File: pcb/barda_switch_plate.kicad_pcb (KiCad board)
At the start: 2 copper layers, 228.6 x 76.2 mm, 4 parts

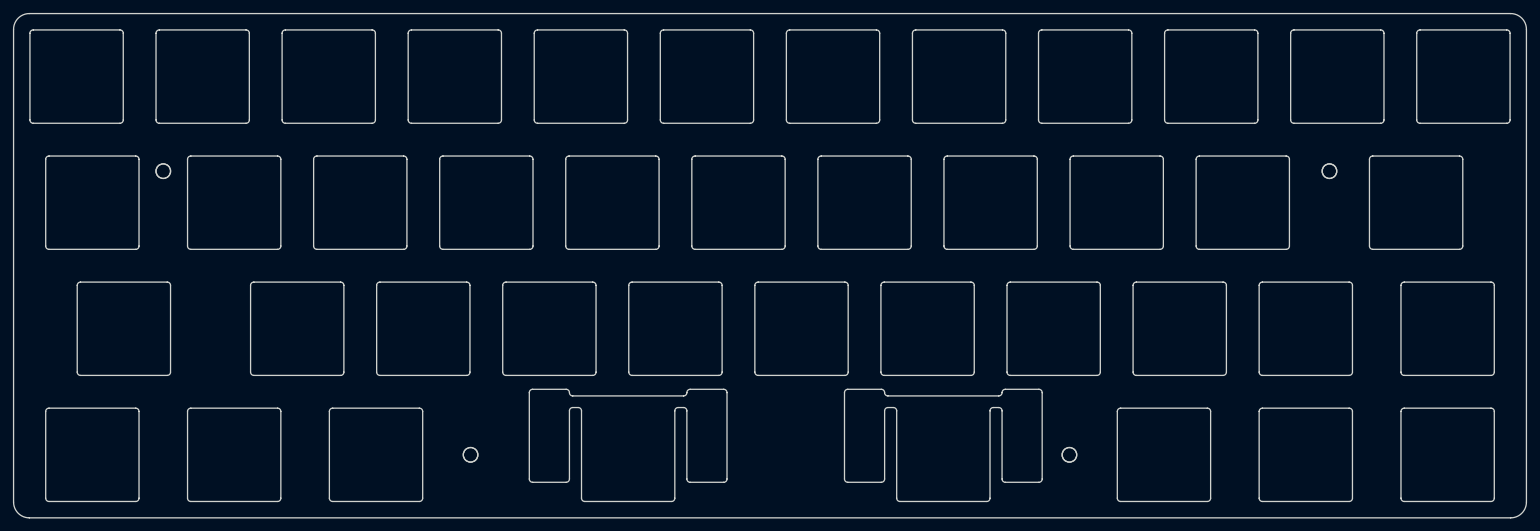
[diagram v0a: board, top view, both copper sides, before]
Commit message: Update Barda case and PCB designs
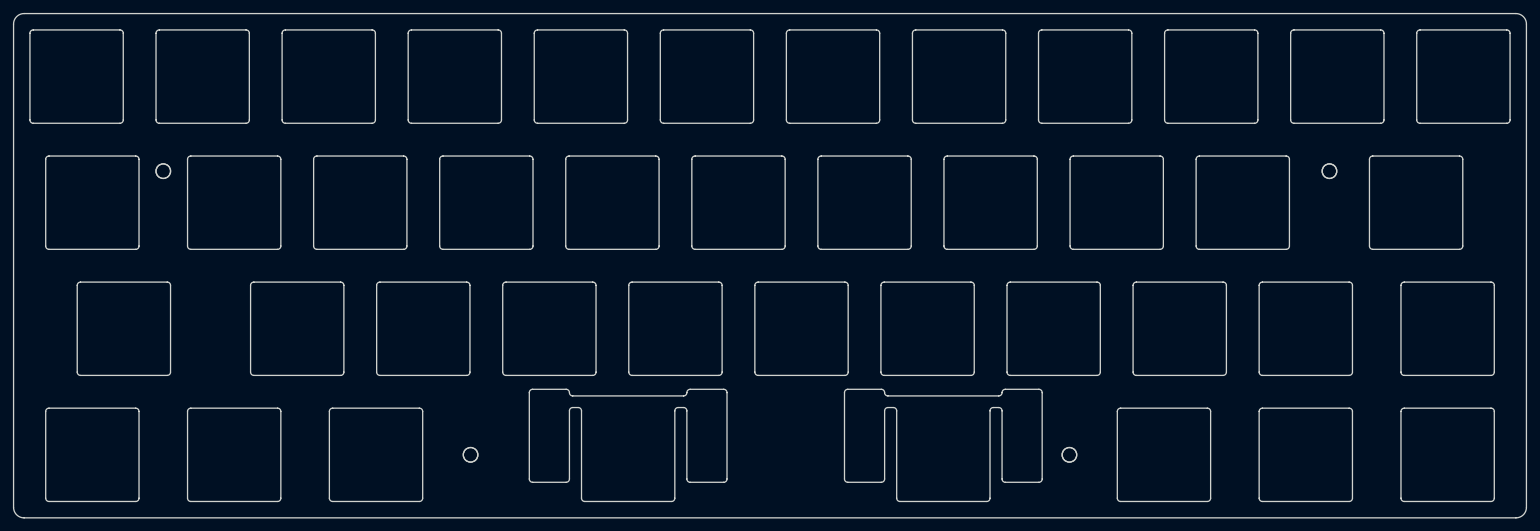
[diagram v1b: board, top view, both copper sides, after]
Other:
- outline, holes or cut-outs redrawn
